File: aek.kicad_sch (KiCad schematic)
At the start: 242 parts, among them J1 Conn_01x04_MountingPin, SW1 SW_Push, U1 ATmega32U4-AU, U2 ATmega32U4-AU, Y1 16MHz

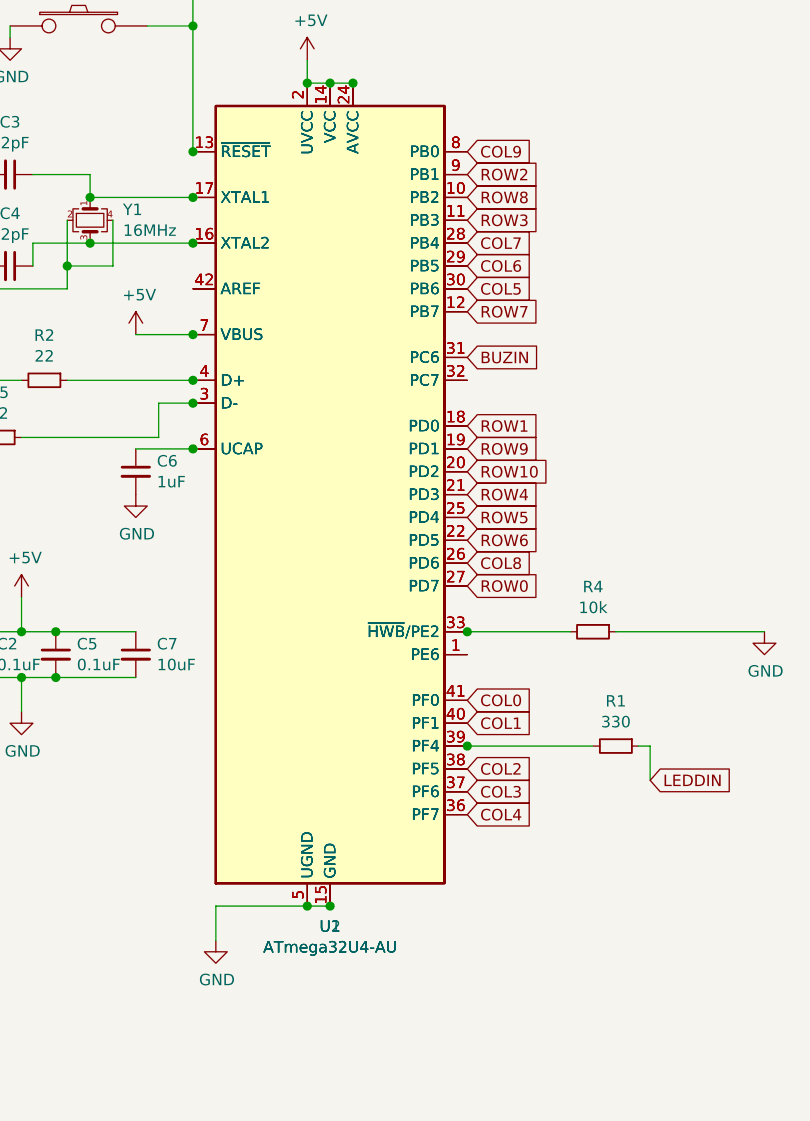
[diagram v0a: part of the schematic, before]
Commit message: updates
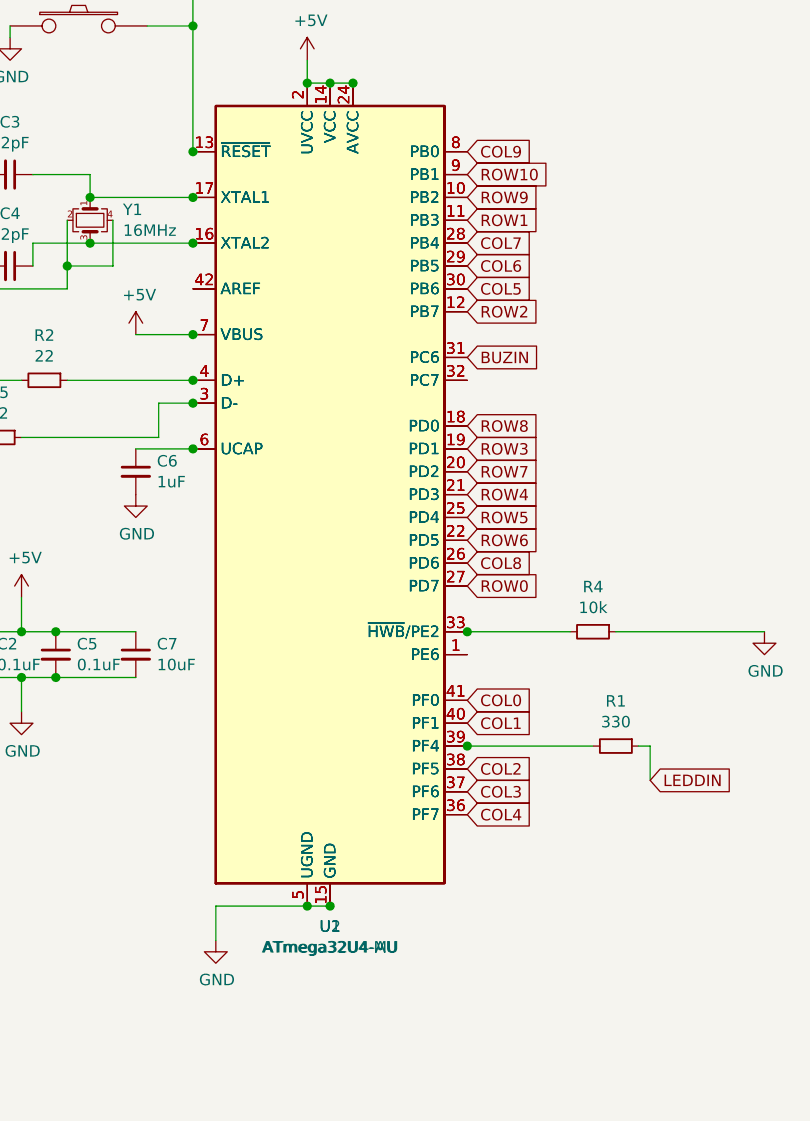
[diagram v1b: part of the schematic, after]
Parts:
- U2: value ATmega32U4-AU -> ATmega32U4-MU
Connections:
- net ROW1: now also U1.11 (PB3), U2.11 (PB3); no longer U1.18 (PD0), U2.18 (PD0)
- net ROW10: now also U1.9 (PB1), U2.9 (PB1); no longer U1.20 (PD2), U2.20 (PD2)
- net ROW2: now also U1.12 (PB7), U2.12 (PB7); no longer U1.9 (PB1), U2.9 (PB1)
- net ROW3: now also U1.19 (PD1), U2.19 (PD1); no longer U1.11 (PB3), U2.11 (PB3)
- net ROW7: now also U1.20 (PD2), U2.20 (PD2); no longer U1.12 (PB7), U2.12 (PB7)
- net ROW8: now also U1.18 (PD0), U2.18 (PD0); no longer U1.10 (PB2), U2.10 (PB2)
- net ROW9: now also U1.10 (PB2), U2.10 (PB2); no longer U1.19 (PD1), U2.19 (PD1)
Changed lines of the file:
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@@
     )
   )
-  (global_label "ROW2" (shape input) (at 87.63 62.23 0) (fields_autoplaced)
+  (global_label "ROW10" (shape input) (at 87.63 62.23 0) (fields_autoplaced)
     (effects (font (size 1.27 1.27)) (justify left))
-    (property "Intersheet References" "${INTERSHEET_REFS}" (id 0) (at 7.62 -41.91 0)
+    (property "Intersheet References" "${INTERSHEET_REFS}" (id 0) (at 7.62 -74.93 0)
       (effects (font (size 1.27 1.27)) hide)
     )
   )
-  (global_label "ROW8" (shape input) (at 87.63 64.77 0) (fields_autoplaced)
+  (global_label "ROW9" (shape input) (at 87.63 64.77 0) (fields_autoplaced)
     (effects (font (size 1.27 1.27)) (justify left))
-    (property "Intersheet References" "${INTERSHEET_REFS}" (id 0) (at 7.62 -41.91 0)
+    (property "Intersheet References" "${INTERSHEET_REFS}" (id 0) (at 7.62 -69.85 0)
       (effects (font (size 1.27 1.27)) hide)
     )
   )
-  (global_label "ROW3" (shape input) (at 87.63 67.31 0) (fields_autoplaced)
+  (global_label "ROW1" (shape input) (at 87.63 67.31 0) (fields_autoplaced)
     (effects (font (size 1.27 1.27)) (justify left))
-    (property "Intersheet References" "${INTERSHEET_REFS}" (id 0) (at 7.62 -41.91 0)
+    (property "Intersheet References" "${INTERSHEET_REFS}" (id 0) (at 7.62 -64.77 0)
       (effects (font (size 1.27 1.27)) hide)
     )
@@
     )
   )
-  (global_label "ROW7" (shape input) (at 87.63 77.47 0) (fields_autoplaced)
+  (global_label "ROW2" (shape input) (at 87.63 77.47 0) (fields_autoplaced)
     (effects (font (size 1.27 1.27)) (justify left))
-    (property "Intersheet References" "${INTERSHEET_REFS}" (id 0) (at 7.62 -41.91 0)
+    (property "Intersheet References" "${INTERSHEET_REFS}" (id 0) (at 7.62 -26.67 0)
       (effects (font (size 1.27 1.27)) hide)
     )
@@
     )
   )
-  (global_label "ROW1" (shape input) (at 87.63 90.17 0) (fields_autoplaced)
+  (global_label "ROW8" (shape input) (at 87.63 90.17 0) (fields_autoplaced)
     (effects (font (size 1.27 1.27)) (justify left))
-    (property "Intersheet References" "${INTERSHEET_REFS}" (id 0) (at 7.62 -41.91 0)
+    (property "Intersheet References" "${INTERSHEET_REFS}" (id 0) (at 7.62 -16.51 0)
       (effects (font (size 1.27 1.27)) hide)
     )
   )
-  (global_label "ROW9" (shape input) (at 87.63 92.71 0) (fields_autoplaced)
+  (global_label "ROW3" (shape input) (at 87.63 92.71 0) (fields_autoplaced)
     (effects (font (size 1.27 1.27)) (justify left))
-    (property "Intersheet References" "${INTERSHEET_REFS}" (id 0) (at 7.62 -41.91 0)
+    (property "Intersheet References" "${INTERSHEET_REFS}" (id 0) (at 7.62 -16.51 0)
       (effects (font (size 1.27 1.27)) hide)
     )
   )
-  (global_label "ROW10" (shape input) (at 87.63 95.25 0) (fields_autoplaced)
+  (global_label "ROW7" (shape input) (at 87.63 95.25 0) (fields_autoplaced)
     (effects (font (size 1.27 1.27)) (justify left))
-    (property "Intersheet References" "${INTERSHEET_REFS}" (id 0) (at 7.62 -41.91 0)
+    (property "Intersheet References" "${INTERSHEET_REFS}" (id 0) (at 7.62 -24.13 0)
       (effects (font (size 1.27 1.27)) hide)
     )
@@
     (in_bom yes) (on_board yes)
     (property "Reference" "U2" (id 0) (at 72.39 145.7706 0))
-    (property "Value" "ATmega32U4-AU" (id 1) (at 72.39 148.082 0))
+    (property "Value" "ATmega32U4-MU" (id 1) (at 72.39 148.082 0))
     (property "Footprint" "Package_DFN_QFN:QFN-44-1EP_7x7mm_P0.5mm_EP5.2x5.2mm" (id 2) (at 72.39 97.79 0)
       (effects (font (size 1.27 1.27) italic) hide)
@@
     )
     (path "/2ccdb65d-62ed-42d5-acea-df4cedf22149"
-      (reference "U2") (unit 1) (value "ATmega32U4-AU") (footprint "Package_DFN_QFN:QFN-44-1EP_7x7mm_P0.5mm_EP5.2x5.2mm")
+      (reference "U2") (unit 1) (value "ATmega32U4-MU") (footprint "Package_DFN_QFN:QFN-44-1EP_7x7mm_P0.5mm_EP5.2x5.2mm")
     )
     (path "/00000000-0000-0000-0000-0000612269b2"
